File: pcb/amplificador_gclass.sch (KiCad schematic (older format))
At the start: 43 parts, among them CON1 AUDIO_IN, P1 +VA_GND, P2 +VB_GND, P3 -VA_GND, P4 -VB_GND, P5 OUT, P6 CONN_01X01, Q1 MPSA56_PNP_EBC, Q10 MPSA06_NPN_EBC, Q11 MPSA56_PNP_EBC, Q12 MPSA06_NPN_EBC, Q2 MPSA56_PNP_EBC, Q3 MPSA06_NPN_EBC, Q4 MPSA56_PNP_EBC, Q5 MPSA06_NPN_EBC, Q6 MPSA56_PNP_EBC, Q7 MPSA56_PNP_EBC, Q8 MPSA56_PNP_EBC, Q9 MPSA56_PNP_EBC

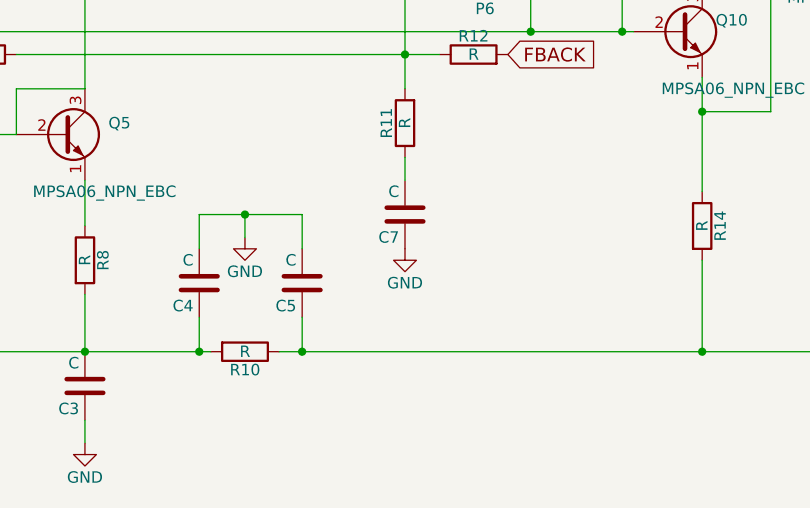
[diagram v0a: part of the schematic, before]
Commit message: ultimos avances falta poco para terminar
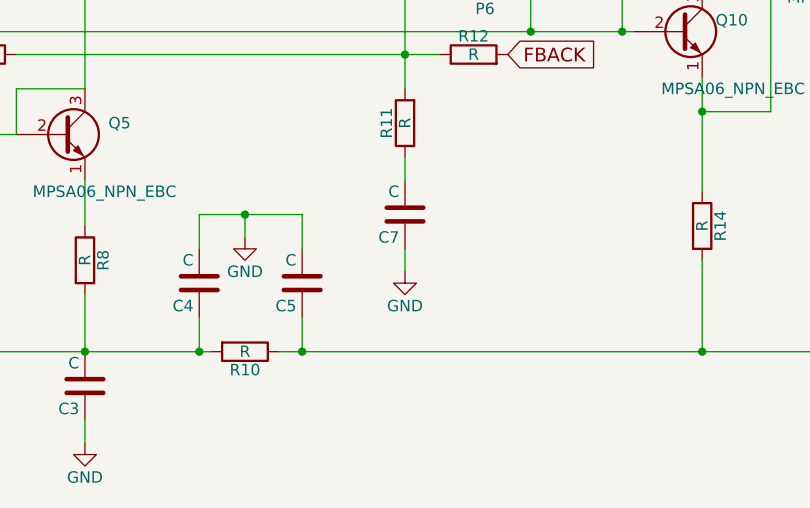
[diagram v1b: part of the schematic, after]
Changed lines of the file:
@@
 L GND #PWR014
 U 1 1 555F1530
-P 6500 5450
-F 0 "#PWR014" H 6500 5200 50  0001 C CNN
-F 1 "GND" H 6500 5300 50  0000 C CNN
-F 2 "" H 6500 5450 60  0000 C CNN
-F 3 "" H 6500 5450 60  0000 C CNN
-	1    6500 5450
+P 6500 5550
+F 0 "#PWR014" H 6500 5300 50  0001 C CNN
+F 1 "GND" H 6500 5400 50  0000 C CNN
+F 2 "" H 6500 5550 60  0000 C CNN
+F 3 "" H 6500 5550 60  0000 C CNN
+	1    6500 5550
 	1    0    0    -1
 $EndComp
@@
 Wire Wire Line
 	5100 6200 5100 6300
+Wire Wire Line
+	6500 5450 6500 5550
 $EndSCHEMATC
